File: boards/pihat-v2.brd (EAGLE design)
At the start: 52.1 x 47.9 mm, 11 parts, among them IC1 2967-MP6500, IC2 2967-MP6500, IC3 2967-MP6500, J10 RASPBERRYPI-40-PIN-GPIO_PTH_N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

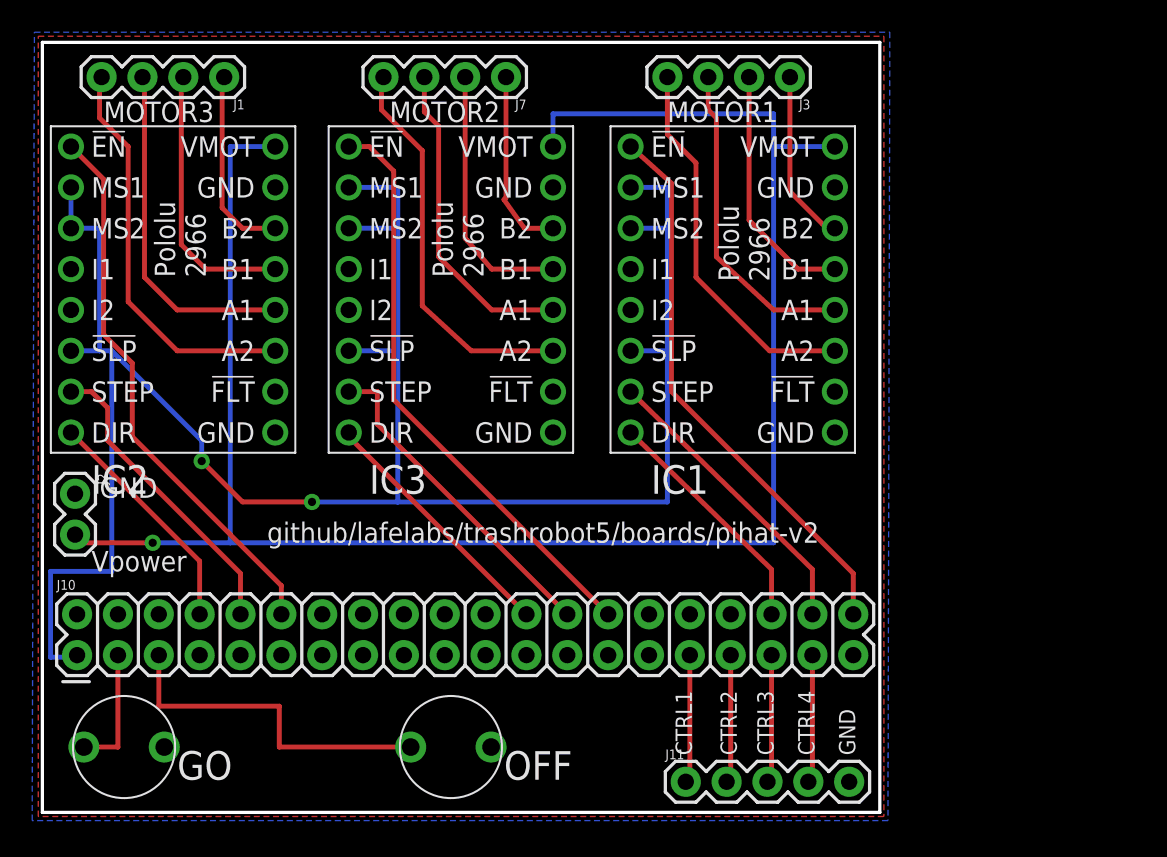
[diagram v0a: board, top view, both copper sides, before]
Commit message: added very useful arduino code
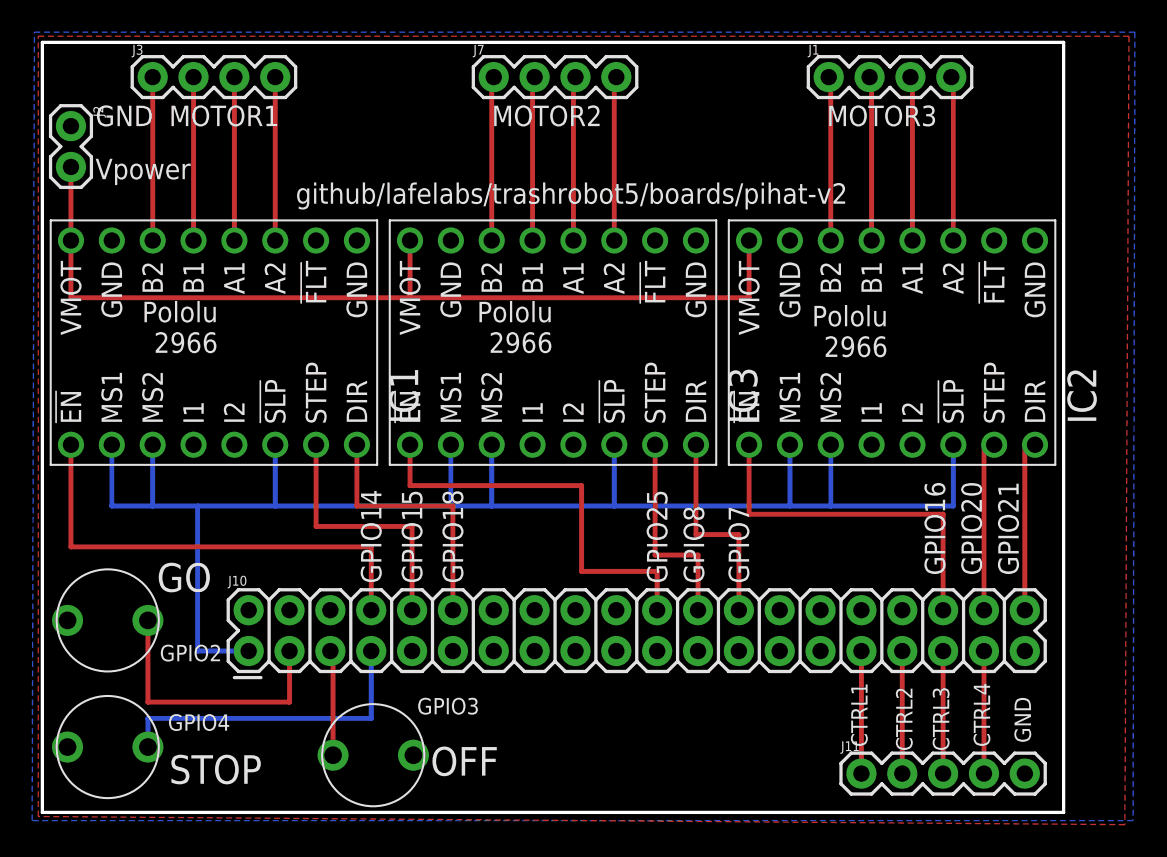
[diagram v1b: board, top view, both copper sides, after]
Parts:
- added U$1: BUTTON, spietz-library-2:BUTTON
- moved IC2 44.8 mm to (52.8, 29.2), turned to 90 degrees
- moved J3 39.6 mm to (6.86, 45.7), turned to 0 degrees
- moved J1 37.6 mm to (48.9, 45.7), turned to 0 degrees
- moved IC1 32.4 mm to (10.7, 29.2), turned to 90 degrees
- moved J2 22.9 mm to (1.78, 42.7)
- moved J11 10.9 mm to (50.9, 2.41)
- moved J10 10.7 mm to (12.8, 10.0)
- moved U$4 7.94 mm to (4.06, 11.9), turned to 180 degrees
- moved IC3 7.16 mm to (31.8, 29.2), turned to 90 degrees
- moved U$5 4.85 mm to (20.6, 3.56)
- moved J7 0.76 mm to (28.1, 45.7), turned to 0 degrees
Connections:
- removed net D25: J10.22
- removed net D4: J10.7
- new net GPIO1: J10.28
- new net STOP: J10.7, U$1.P$1
- net DIR1: now also J10.12; no longer J10.36
- net DIR2: now also J10.26; no longer J10.24
- net DIR3: now also J10.40; no longer J10.8
- net EN1: now also J10.8; no longer J10.40
- net EN2: now also J10.22; no longer J10.28
- net EN3: now also J10.36; no longer J10.12
- net GND: now also U$1.P$2
- net STEP1: now also J10.10; no longer J10.38
- net STEP2: now also J10.24; no longer J10.26
- net STEP3: now also J10.38; no longer J10.10
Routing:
- net 12V: track 117.6 -> 57.4 mm, vias 1 -> 0
- net 3.3V: track 133.3 -> 98.8 mm, vias 2 -> 0
- net STOP: track 0.00 -> 19.9 mm
- net N$12: track 25.2 -> 10.3 mm
- net OFF-GPIO3: track 21.4 -> 6.64 mm
- net N$14: track 24.5 -> 10.3 mm
- net N$8: track 23.7 -> 10.2 mm
- net EN3: track 34.5 -> 22.4 mm
- net N$11: track 21.5 -> 10.3 mm
- net EN2: track 36.5 -> 25.7 mm
- net N$7: track 20.0 -> 10.2 mm
- net N$13: track 20.0 -> 10.3 mm
- net GO-GPIO2: track 7.83 -> 17.1 mm
- net STEP3: track 19.0 -> 10.9 mm
- net STEP2: track 20.5 -> 13.0 mm
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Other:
- board size 52.1 x 47.9 mm -> 63.5 x 47.9 mm
- board text added: "GPIO14"
- board text added: "GPIO15"
- board text added: "GPIO16"
- board text added: "GPIO18"
- board text added: "GPIO2"
- board text added: "GPIO20"
- board text added: "GPIO21"
- board text added: "GPIO25"
- board text added: "GPIO3"
- board text added: "GPIO4"
- board text added: "GPIO7"
- board text added: "GPIO8"
- board text added: "STOP"
